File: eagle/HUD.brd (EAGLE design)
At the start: 72.1 x 47 mm, 61 parts, among them IC1 ATMEGA644A, IC2 LM2576, J1 AVR_SPI, X1 16 MHz, Y3 4MHz

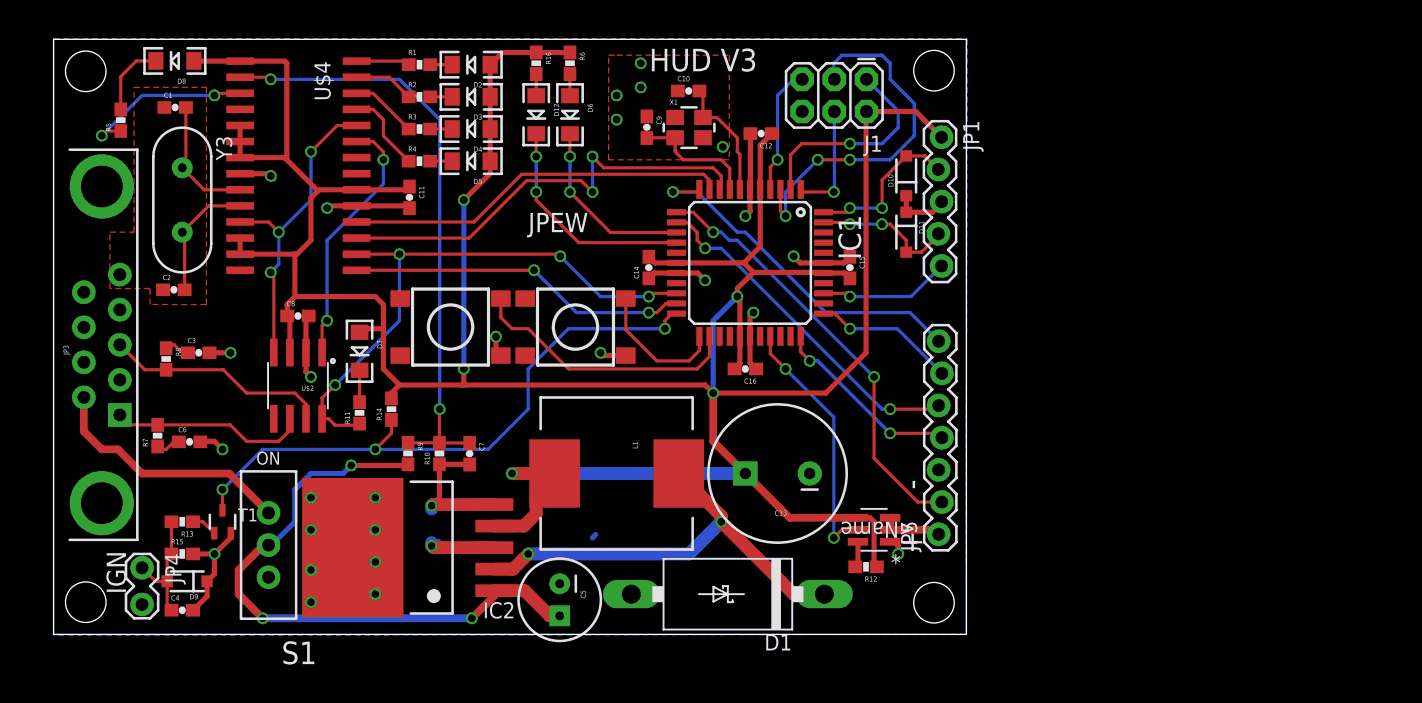
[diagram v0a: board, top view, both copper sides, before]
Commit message: V4 Schematic and board layout
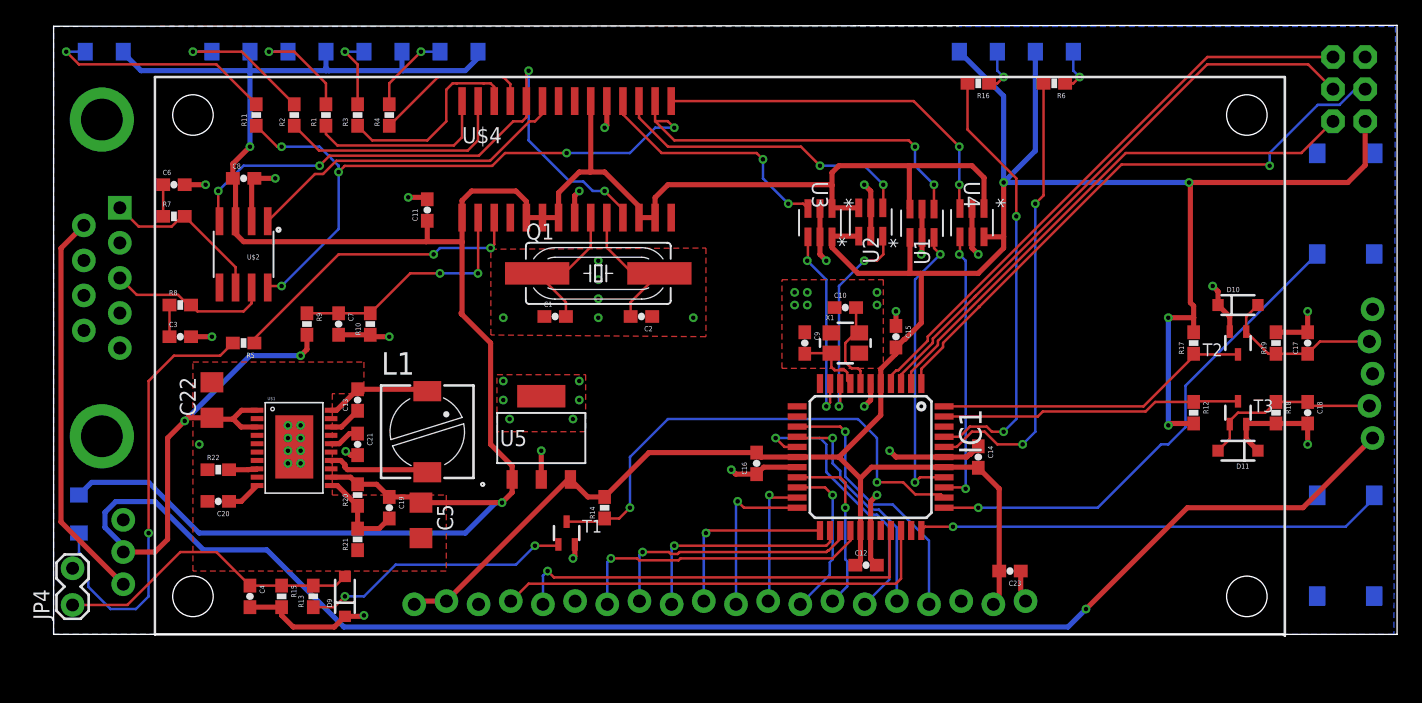
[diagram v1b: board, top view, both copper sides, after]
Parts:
- removed D1: 1N5822, diode:DO201T15
- removed IC2: LM2576, AWJLEagleLib:TO263-5
- removed JP5: DISPLAY, SparkFun-Connectors:1X07_LOCK
- removed Y3: 4MHz, SparkFun-FreqCtrl:HC49US
- added C17, C18, C20, C23: 0.1uF, SparkFun-Capacitors:0603-CAP
- added C19: 4.7pF, SparkFun-Capacitors:0603-CAP
- added C21: 2.2uF, SparkFun-Capacitors:0603-CAP
- added C22: 2.2uF, resistor:C1206
- added J2: (no value), SparkFun-Connectors:1X20_LOCK
- added Q1: 4MHz, crystal:SM49
- added R17, R18, R19: 20K, SparkFun-Passives:0603-RES
- added R20: 1M, SparkFun-Passives:0603-RES
- added R21: 191K, SparkFun-Passives:0603-RES
- added R22: 25.5K, SparkFun-Passives:0603-RES
- added T2, T3: (no value), zetex:SOT323
- added U1, U2, U3, U4: SN74LVC1T45DBVR, MyLibrary:DBV6
- added U5: MCP1825S-3002E/DB, MyLibrary:SOT-223_3MC
- C13: value 680uF -> 0.1uF; device SparkFun-Capacitors:CPOL-RADIAL-1000UF-25V -> SparkFun-Capacitors:0603-CAP
- C5: value 100uF -> 47uF; device SparkFun-Capacitors:CPOL-RADIAL-100UF-25V -> resistor:C1206
- D10, D11: value 7V -> 24V
- L1: value 150uH -> 22uH; device SparkFun-Passives:CDRH125 -> rcl:PIS2816
- R12: value 127K -> 20K
- R16, R6: value 470 -> 34
- U$1: value TPS27082LDDCRDDC6-M -> LT8631; device power:DDC6-M -> MyLibrary:TSSOP20
- X1: value 16 MHz -> 10 MHz
- moved S4 72.7 mm to (102.0, 7.00), flipped to the bottom, turned to 90 degrees
- moved S2 61.6 mm to (102.0, 34.0), flipped to the bottom, turned to 270 degrees
- moved U$1 46.3 mm to (19.0, 15.0), turned to 0 degrees
- moved JP1 41.5 mm to (104.0, 15.5), flipped to the bottom, turned to 90 degrees
- moved D6 38.6 mm to (79.0, 46.0), flipped to the bottom, turned to 180 degrees
- moved R6 38.3 mm to (79.0, 43.5), turned to 180 degrees
- moved J1 37.0 mm to (101.0, 40.5), flipped to the bottom, turned to 90 degrees
- moved C2 37.0 mm to (46.4, 25.1), turned to 180 degrees
- moved D8 36.6 mm to (2.00, 9.50), flipped to the bottom, turned to 270 degrees
- moved D12 35.3 mm to (73.0, 46.0), flipped to the bottom, turned to 180 degrees
- moved C12 35.1 mm to (64.1, 5.46), turned to 0 degrees
- moved R16 34.9 mm to (73.0, 43.5), turned to 180 degrees
- moved C1 34.2 mm to (39.6, 25.1)
- moved C13 33.7 mm to (24.0, 18.5), turned to 90 degrees
- moved D11 31.4 mm to (93.5, 14.5), turned to 180 degrees
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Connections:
- removed net DISPLAY_BUSY: IC1.33, JP5.4
- removed net EXT_SLEEP: IC1.36, JP1.5
- removed net N$26: D6.A, R6.2
- removed net VCC_VFD: JP5.1, U$1.2, U$1.3
- removed net VFD_ON: IC1.30, U$1.5
- removed net VFD_RESET: IC1.34, JP5.6
- new net AVR_TO_ELM_3: IC1.10, U3.4
- new net C/S_1: IC1.31, J2.17
- new net C/S_2: IC1.32
- new net D/C: IC1.14, J2.4
- new net D0: IC1.19, J2.7
- new net D1: IC1.20, J2.8
- new net D2: IC1.21, J2.9
- new net D3: IC1.22, J2.10
- new net D4: IC1.23, J2.11
- new net D5: IC1.24, J2.12
- new net D6: IC1.25, J2.13
- new net D7: IC1.26, J2.14
- new net E: IC1.16, J2.6
- new net ELM_TO_AVR_3: IC1.9, U2.3
- new net N$12: C17.1, D10.A, JP1.4, R19.1, T2.2
- new net N$13: C18.1, D11.A, JP1.2, R18.1, T3.2
- new net N$23: C13.2, L1.1, U$1.20
- new net N$24: C13.1, U$1.18
- new net N$25: C20.1, U$1.10
- new net N$27: C19.2, R20.1, R21.2, U$1.11
- new net N$31: C21.1, U$1.16
- new net N$34: R22.2, U$1.8
- new net POWER_CTRL_3: IC1.37, U1.3
- new net R/W: IC1.15, J2.5
- new net RES: IC1.30, J2.16
- new net RTS_IGNMON_3: IC1.36, U4.4
- new net VCC_2: C12.1, C14.2, C15.2, C16.2, C23.2, D12.A, D6.A, IC1.17, IC1.27, IC1.38, IC1.5, J1.2, J2.19, J2.2, J2.20, R12.2, R14.2, R17.2, U1.1, U2.1, U3.6, U4.6, U5.3
- net AVR_TO_DISPLAY: no longer JP5.2
- net AVR_TO_ELM: now also U3.3; no longer IC1.10
- net BTN_LEFT: now also IC1.33; no longer IC1.24
- net BTN_LEFT_EXT: now also R17.1, T2.1; no longer D10.A, JP1.2
- net BTN_RIGHT: now also IC1.34; no longer IC1.23
- net BTN_RIGHT_EXT: now also R12.1, T3.1; no longer D11.A, JP1.4
- net DISPLAY_CLOCK: no longer JP5.5
- net DISPLAY_TO_AVR: no longer JP5.7
- net ELM_TO_AVR: now also U2.4; no longer IC1.9
- net GND: now also C17.2, C18.2, C20.2, C21.2, C22.2, C23.1, J2.1, R18.2, R19.2, R21.1, R22.1, T2.3, T3.3, U$1.21, U$1.7, U1.2, U1.5, U2.2, U2.5, U3.2, U3.5, U4.2, U4.5, U5.2, U5.4; no longer C13.-, D1.A, IC2.3, IC2.5, IC2.TAB, JP5.3, U$1.1
- net IGNMON: now also IC1.35; no longer IC1.22
- net N$1: now also D12.C, R16.1; no longer R12.2, U$1.6
- net N$10: now also D6.C, R6.1; no longer D12.C, IC1.15
- net N$15: now also Q1.1; no longer Y3.1
- net N$16: now also Q1.2; no longer Y3.2
- net N$4: now also IC1.40, R6.2; no longer D6.C, IC1.14
- net N$6: now also L1.2, U$1.14; no longer D1.C, IC2.2, L1.1
- net N$8: now also IC1.41; no longer D12.A
- net POWER_CTRL: now also U1.4; no longer IC1.20
- net RTS_IGNMON: now also U4.3; no longer IC1.21
- net VCC: now also C19.1, C5.1, R20.2, U$1.12, U1.6, U2.6, U3.1, U4.1, U5.1; no longer C12.1, C13.+, C14.2, C15.2, C16.2, IC1.17, IC1.27, IC1.38, IC1.5, IC2.4, J1.2, JP1.1, L1.2, R12.1, R14.2, R16.1, R6.1, U$1.4
- net V_BATT: now also C22.1, JP1.1, U$1.1, U$1.3; no longer C5.1, IC2.1
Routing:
- net VCC_2: track 0.00 -> 195.8 mm, vias 0 -> 4
- net V_BATT: track 48.3 -> 149.7 mm
- net VCC: track 262.9 -> 211.3 mm, vias 5 -> 2
- net MOSI: track 9.06 -> 46.4 mm
- net RESET: track 10.1 -> 46.1 mm, vias 1 -> 0
- net C/S_1: track 0.00 -> 35.3 mm
- net AVR_TO_DISPLAY: track 34.2 -> 0.00 mm, vias 2 -> 0
- net RES: track 0.00 -> 33.7 mm, vias 0 -> 1
- net N$8: track 1.71 -> 34.7 mm, vias 0 -> 2
- net POWER_CTRL: track 45.5 -> 78.5 mm, vias 4 -> 7
- net N$22: track 5.88 -> 35.3 mm, vias 0 -> 1
- net BTN_RIGHT: track 10.8 -> 39.7 mm, vias 0 -> 1
- net N$32: track 47.5 -> 19.2 mm
- net DISPLAY_TO_AVR: track 28.0 -> 0.00 mm, vias 1 -> 0
- net DISPLAY_CLOCK: track 27.3 -> 0.00 mm, vias 2 -> 0
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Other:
- board size 72.1 x 47 mm -> 106.1 x 48.1 mm
- board text added: "HUD V4"
- board text removed: "+"
- board text removed: "-"
- board text removed: "HUD V3"
- board text removed: "IGN"
- board text removed: "ON"
